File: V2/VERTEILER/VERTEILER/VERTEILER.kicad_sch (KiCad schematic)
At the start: 13 parts, among them J1 Conn_01x03, J2 Conn_01x03, J3 Conn_01x03, J4 Conn_01x03, J5 Conn_01x03, Q3 QM6006D

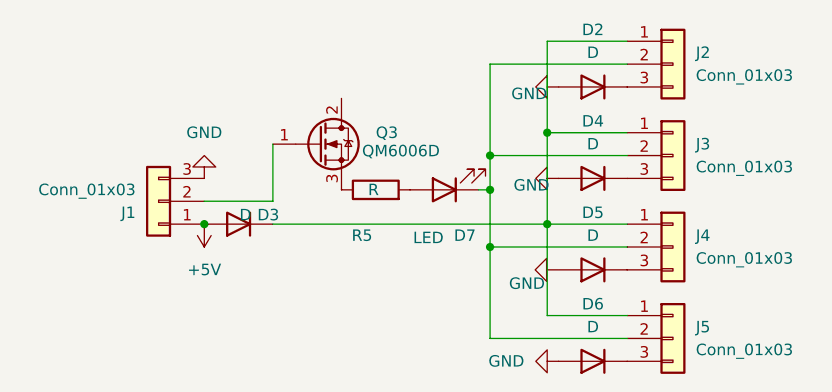
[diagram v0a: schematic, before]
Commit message: Auto-update: 15.04.2026 12:54:54,95
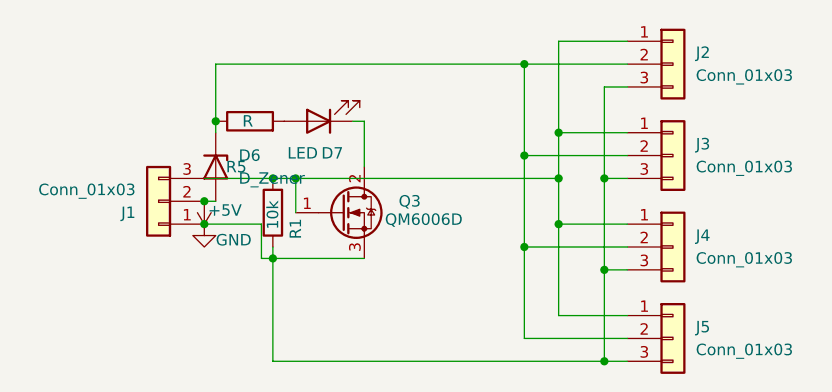
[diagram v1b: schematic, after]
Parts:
- removed D2, D3, D4, D5, D6: D, symbol Device:D
- added D6: D_Zener, Diode_SMD:D_0201_0603Metric, symbol Device:D_Zener
- added R1: 10k, Resistor_SMD:R_1206_3216Metric, symbol Device:R
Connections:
- net +5V: now also J1.2 (Pin_2), D6.2 (A); no longer J1.1 (Pin_1)
- net GND: now also J1.1 (Pin_1), J2.3 (Pin_3), J3.3 (Pin_3), J4.3 (Pin_3), J5.3 (Pin_3), Q3.3 (S), R1.1; no longer J1.3 (Pin_3)
- net at J2.1 (Pin_1), J3.1 (Pin_1), J4.1 (Pin_1)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: now also J1.3 (Pin_3), Q3.1 (G), R1.2
- net at J2.2 (Pin_2), J3.2 (Pin_2), J4.2 (Pin_2)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: now also R5.1, D6.1 (K); no longer D7.1 (K)
- net at Q3.2 (D): now also D7.1 (K)
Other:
- moved on the sheet: D7, Q3, R5
